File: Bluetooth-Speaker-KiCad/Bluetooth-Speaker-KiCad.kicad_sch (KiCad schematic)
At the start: 28 parts, among them J1 Screw_Terminal_01x02, J2 USB_C_Receptacle_USB2.0_14P, Q1 Q_PMOS_DSG, SW1 SW_Push, SW2 SW_Push, U1 RT6150B-33GQW, U2 MAX98357A, U4 TPD4E02B04DQA, U5 ESP32-C3-WROOM-02, U6 MAX1811

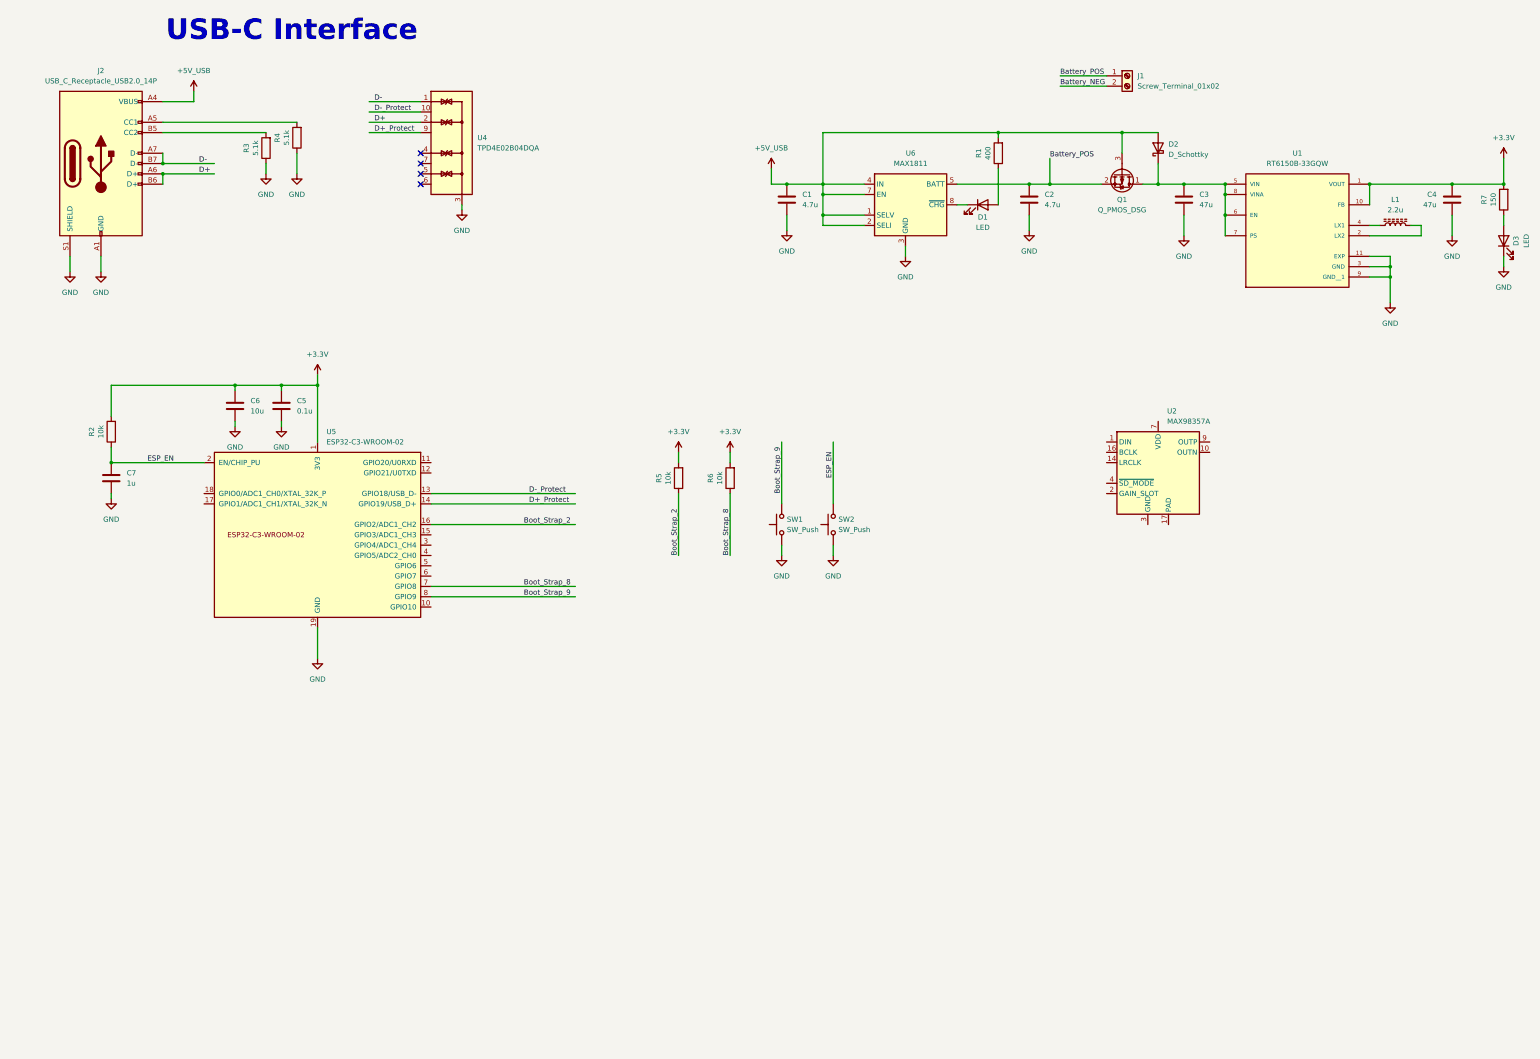
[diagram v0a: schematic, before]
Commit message: Updated schematic
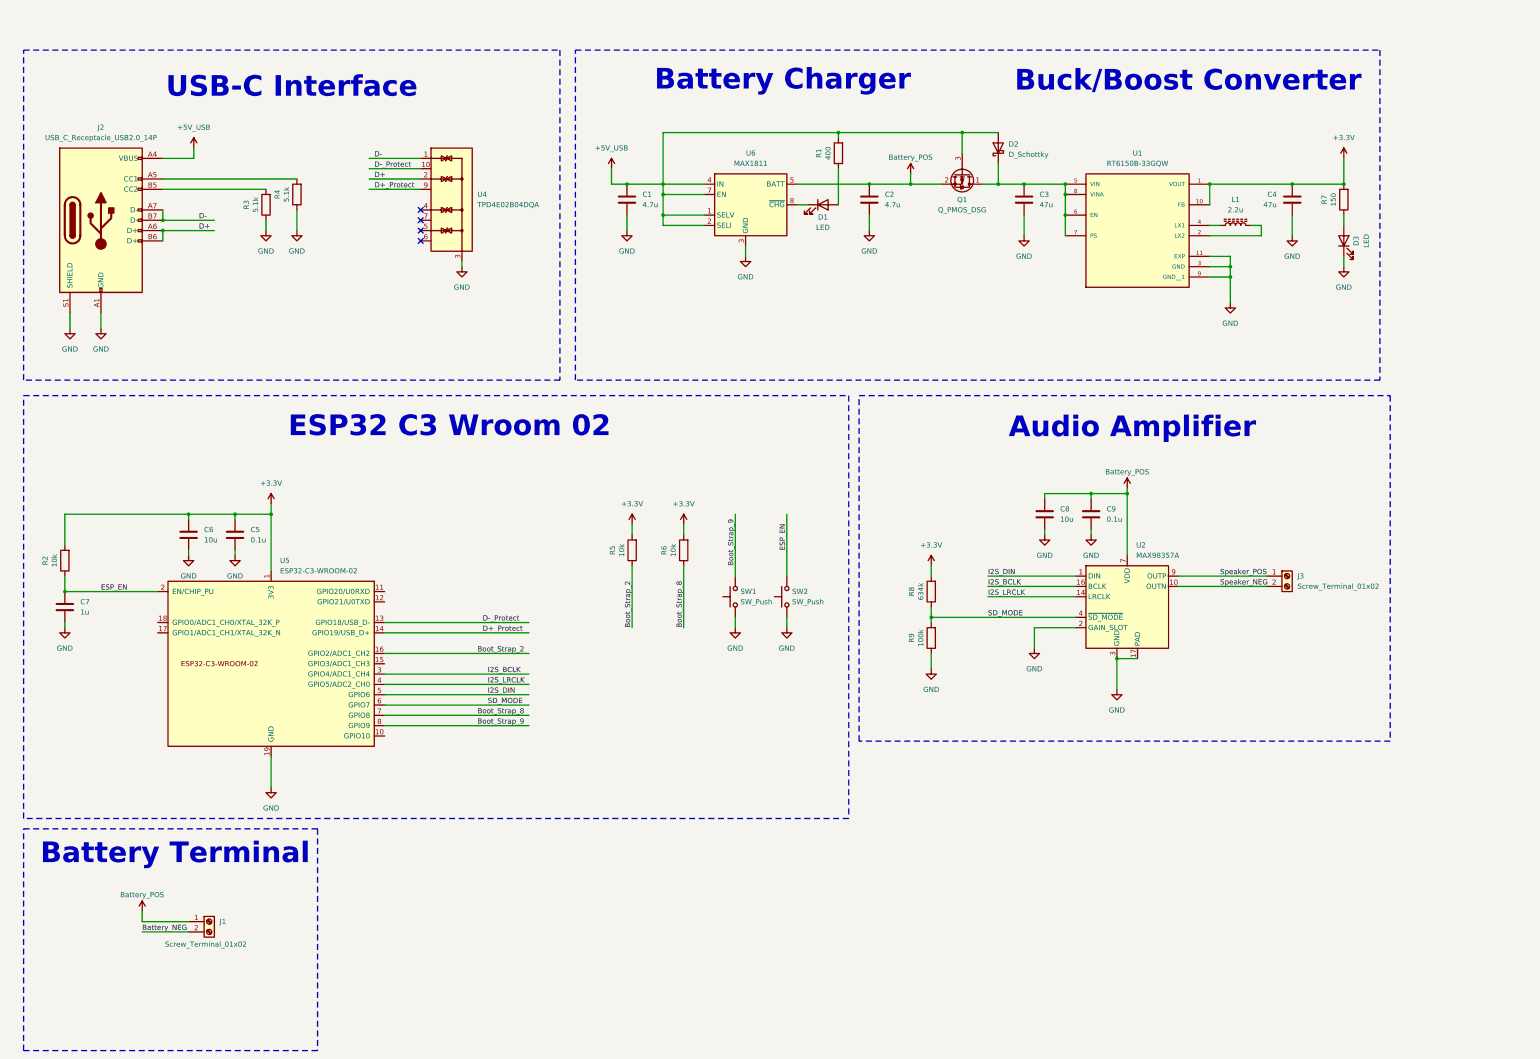
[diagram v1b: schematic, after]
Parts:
- added C8: 10u, Capacitor_SMD:C_0603_1608Metric_Pad1.08x0.95mm_HandSolder, symbol Device:C
- added C9: 0.1u, Capacitor_SMD:C_0603_1608Metric_Pad1.08x0.95mm_HandSolder, symbol Device:C
- added J3: Screw_Terminal_01x02, symbol Connector:Screw_Terminal_01x02
- added R8: 634k, Resistor_SMD:R_0603_1608Metric_Pad0.98x0.95mm_HandSolder, symbol Device:R
- added R9: 100k, Resistor_SMD:R_0603_1608Metric_Pad0.98x0.95mm_HandSolder, symbol Device:R
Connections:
- net +3.3V: now also R8.2
- net Battery_POS: now also U2.7 (VDD), U2.8 (VDD), C8.1, C9.1
- net GND: now also U2.11 (GND), U2.15 (GND), U2.17 (PAD), U2.2 (GAIN_SLOT), U2.3 (GND), C8.2, C9.2, R9.1
- net I2S_BCLK: now reaches U5.3 (GPIO4/ADC1_CH4)
- net I2S_BCLK: now also U2.16 (BCLK)
- net I2S_LRCLK: now reaches U5.4 (GPIO5/ADC2_CH0)
- net I2S_LRCLK: now also U2.14 (LRCLK)
- net I2S_DIN: now reaches U5.5 (GPIO6)
- net I2S_DIN: now also U2.1 (DIN)
- net SD_MODE: now reaches U5.6 (GPIO7)
- net SD_MODE: now also U2.4 (~{SD_MODE}), R8.1, R9.2
- net Speaker_NEG: now reaches U2.10 (OUTN)
- net Speaker_NEG: now also J3.2 (Pin_2)
- net Speaker_POS: now reaches U2.9 (OUTP)
- net Speaker_POS: now also J3.1 (Pin_1)
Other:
- note added: "Audio Amplifier"
- note added: "Battery Charger"
- note added: "Battery Terminal"
- note added: "Buck/Boost Converter"
- note added: "ESP32 C3 Wroom 02"
- moved on the sheet: C1, C2, C3, C4, C5, C6, C7, D1, D2, D3, J1, J2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
